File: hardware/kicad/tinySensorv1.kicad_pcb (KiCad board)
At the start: 2 copper layers, 91.2 x 57.7 mm, 18 parts, among them J1 RADIO, J10 CR2032 socket, J11 AAA socket, J12 AA Socket, J13 Bornier, J2 DCDC converter, J3 BMP/BME breakout, J5 OneWire sensor, J6 ISP, J7 Analog sensor, U1 ATtiny84A-PU

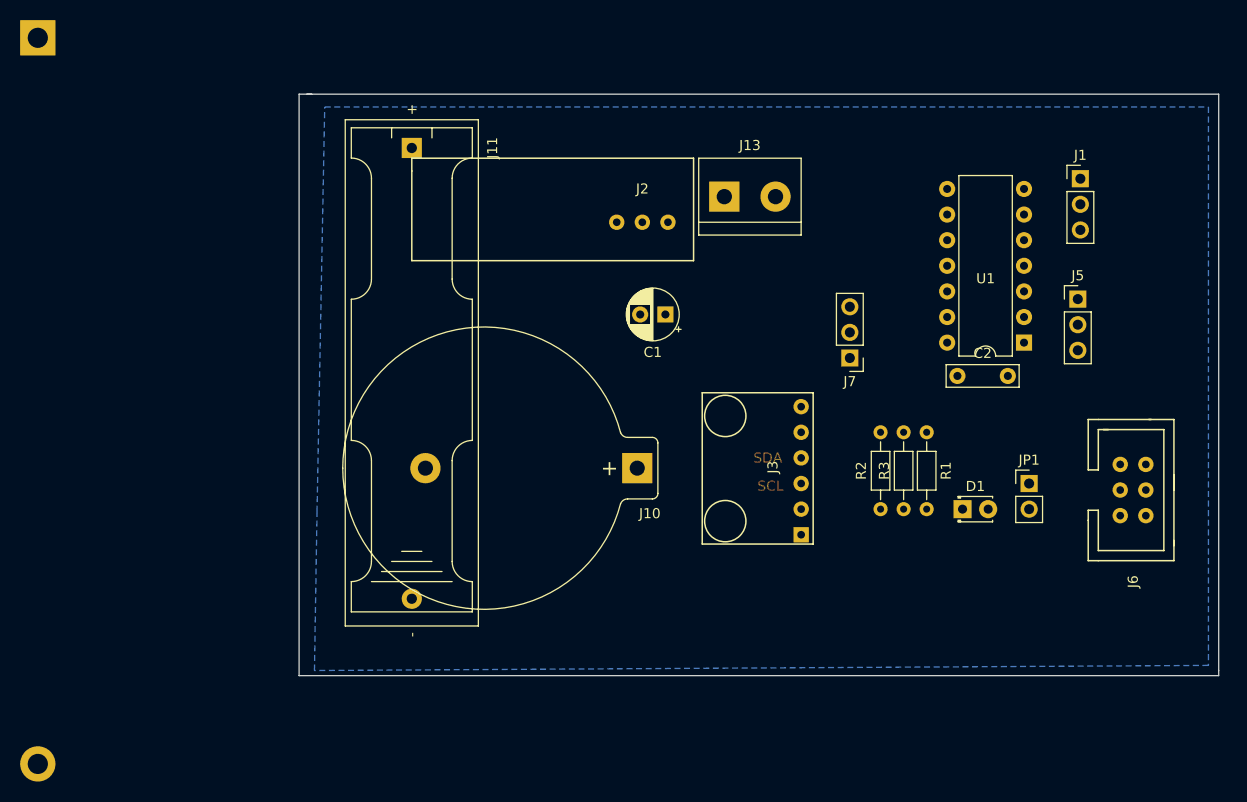
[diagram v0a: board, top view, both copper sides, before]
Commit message: Finish a first version of PCB layout
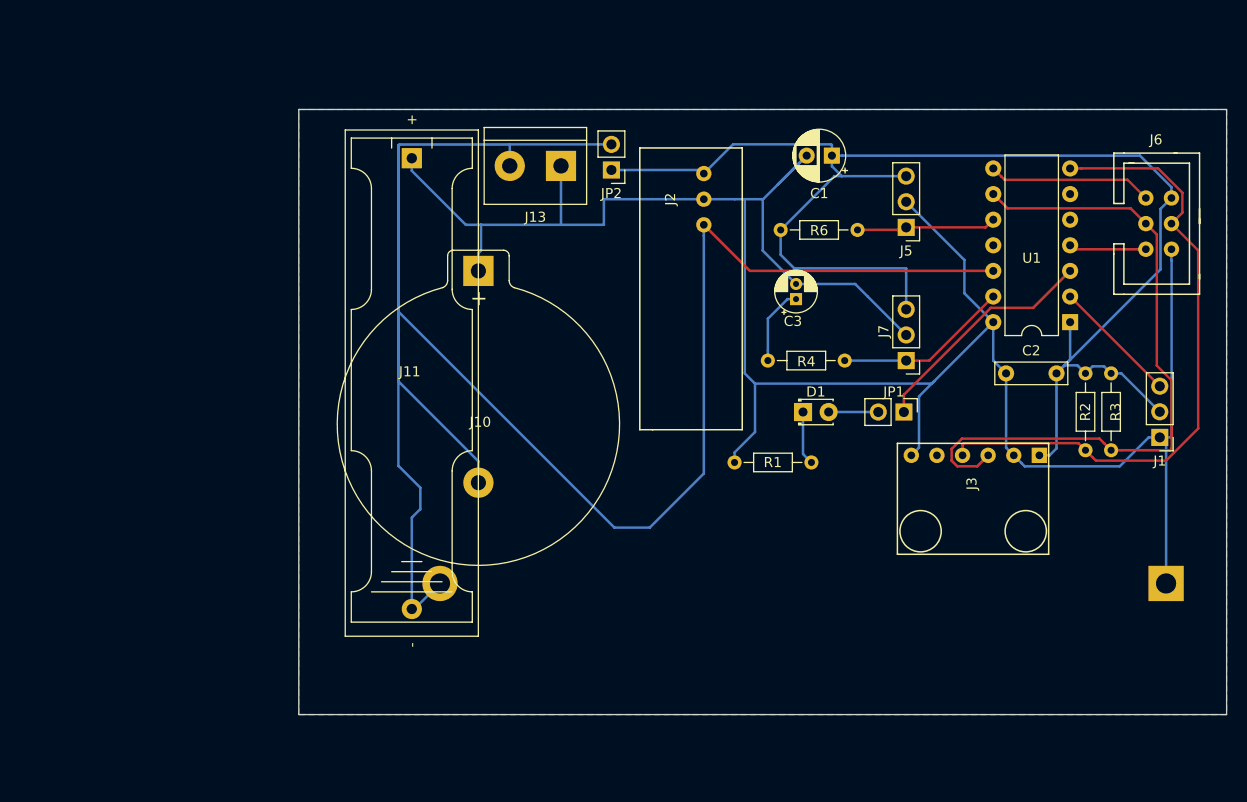
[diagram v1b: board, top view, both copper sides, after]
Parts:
- added C3: 1u, Capacitor_THT:CP_Radial_D4.0mm_P1.50mm, F.Cu at (162.3, 66.8)
- added JP2: Direct alim, Connector_PinHeader_2.54mm:PinHeader_1x02_P2.54mm_Vertical, F.Cu at (144.0, 54.0)
- added R4: 75R, Resistor_THT:R_Axial_DIN0204_L3.6mm_D1.6mm_P7.62mm_Horizontal, F.Cu at (167.1, 72.9)
- added R6: 4k7, Resistor_THT:R_Axial_DIN0204_L3.6mm_D1.6mm_P7.62mm_Horizontal, F.Cu at (160.8, 59.9)
- moved J12 124.3 mm to (199.0, 95.0), turned to 180 degrees
- moved J1 26.8 mm to (198.4, 80.5), turned to 180 degrees
- moved J6 26.5 mm to (194.8, 52.3)
- moved J10 25.1 mm to (130.8, 64.0), turned to 270 degrees
- moved R3 24.6 mm to (193.5, 74.2), turned to 270 degrees
- moved R2 24.4 mm to (191.0, 74.2), turned to 270 degrees
- moved C1 22.8 mm to (165.9, 52.6)
- moved J3 22.4 mm to (181.4, 86.1), turned to 180 degrees
- moved R1 19.3 mm to (156.2, 83.0), turned to 0 degrees
- moved D1 18.5 mm to (163.0, 78.0)
- moved J5 18.4 mm to (173.2, 59.7), turned to 180 degrees
- moved J13 16.5 mm to (139.0, 53.6), turned to 180 degrees
- moved JP1 14.3 mm to (173.0, 78.0), turned to 270 degrees
- moved J7 5.59 mm to (173.2, 72.9)
- moved U1 5.00 mm to (189.5, 69.1)
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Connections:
- U1 pad 2: Net-(U1-Pad2) -> /TX_RADIO
- U1 pad 6: /TX_RADIO -> /PWM_OUT
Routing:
- net GND: track 0.00 -> 228.4 mm
- net +BATT: track 0.00 -> 224.3 mm
- net +3V3: track 0.00 -> 146.1 mm
- net /SCL: track 0.00 -> 68.0 mm
- net /SDA: track 0.00 -> 63.6 mm
- net /LED_OUT: track 0.00 -> 23.3 mm
- net /Analog_sensor: track 0.00 -> 17.4 mm
- net /MISO: track 0.00 -> 16.3 mm
- net /OneWire: track 0.00 -> 13.9 mm
- net /TX_RADIO: track 0.00 -> 12.6 mm
- net Net-(C3-Pad1): track 0.00 -> 7.75 mm
- net /RESET: track 0.00 -> 7.67 mm
- net Net-(D1-Pad1): track 0.00 -> 5.34 mm
- net Net-(D1-Pad2): track 0.00 -> 4.92 mm
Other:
- board size 91.2 x 57.7 mm -> 92 x 60 mm
- board text removed: "SCL"
- board text removed: "SDA"
